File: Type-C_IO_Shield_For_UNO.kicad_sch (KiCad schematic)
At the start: 40 parts, among them J1 USB_C_Receptacle_USB2.0, J10 Conn_01x04, J11 Conn_01x04, J12 Conn_01x04, J13 Conn_01x04, J14 Conn_01x04, J15 Conn_01x04, J16 Conn_Alalog, J17 Conn_01x06, J18 Conn_01x06, J19 Conn_01x06, J2 Conn_01x04, J20 Conn_Digital, J21 Conn_01x04, J22 Conn_01x04, J23 Conn_IIC, J24 Conn_COM, J25 Conn_URF, J26 Conn_SD, J27 Conn_Bluetooth, J28 Screw_Terminal_01x02, J3 Conn_01x04, J4 Conn_01x04, J5 Conn_01x04, J6 Conn_01x04, J7 Conn_01x04, J8 Conn_Digital_2, J9 Conn_Power, U1 CH340C

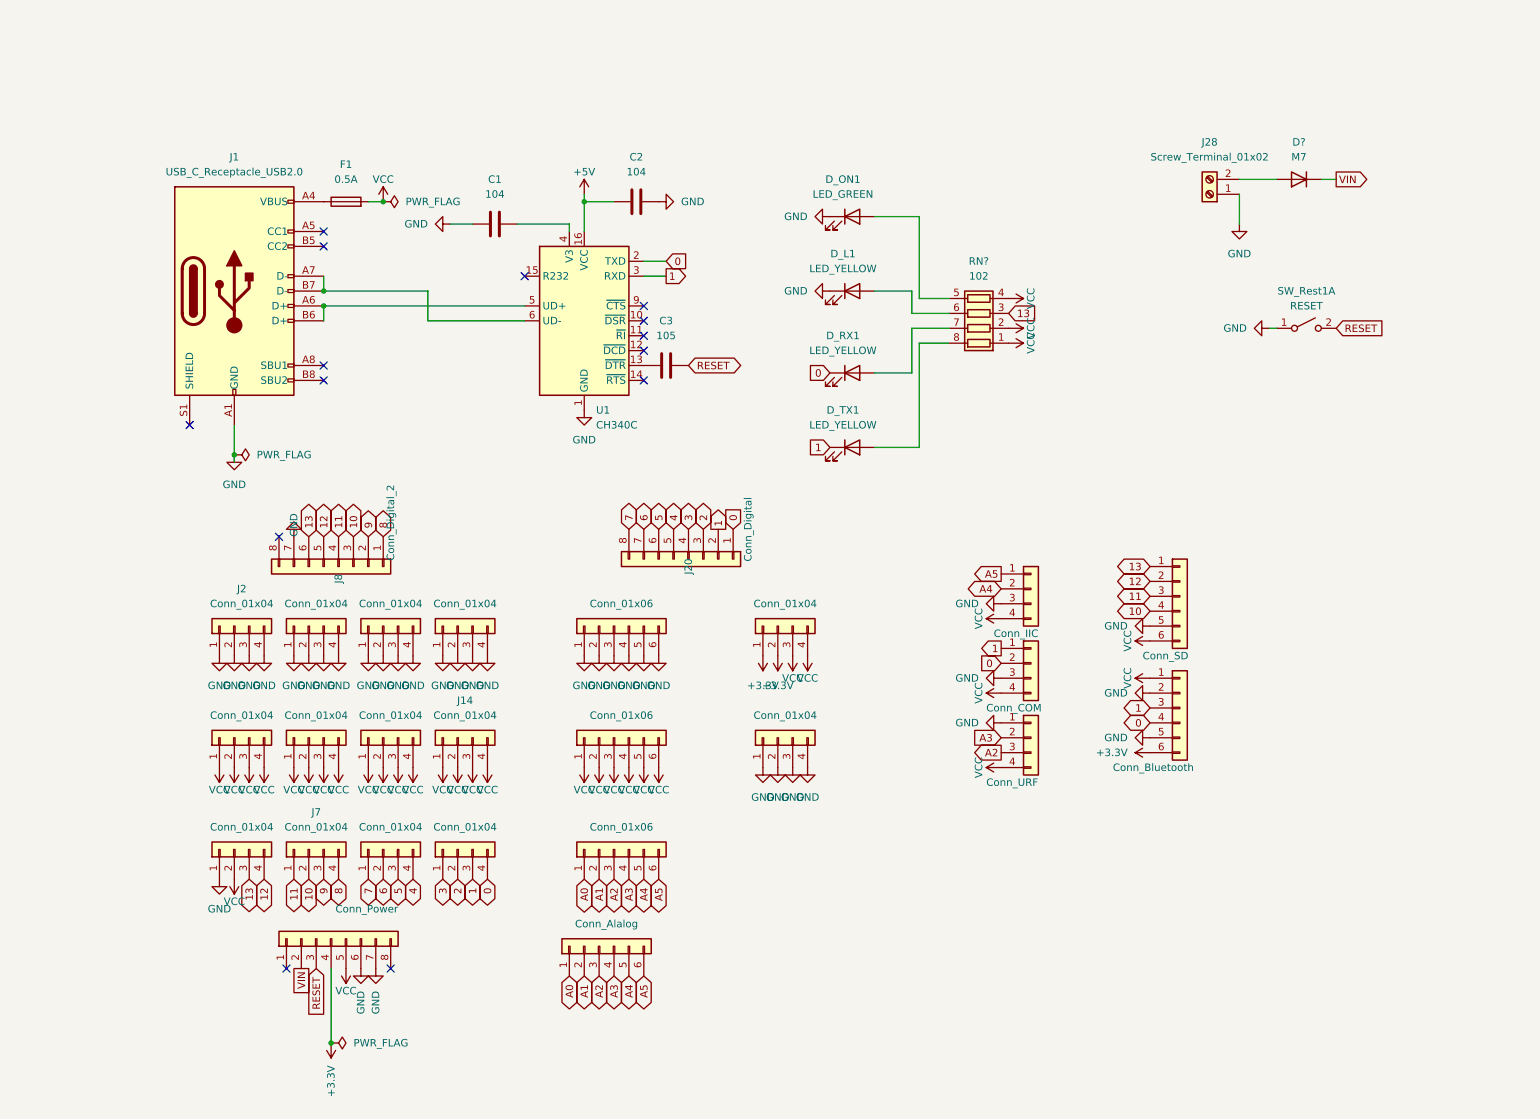
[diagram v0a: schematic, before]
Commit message: V1.1
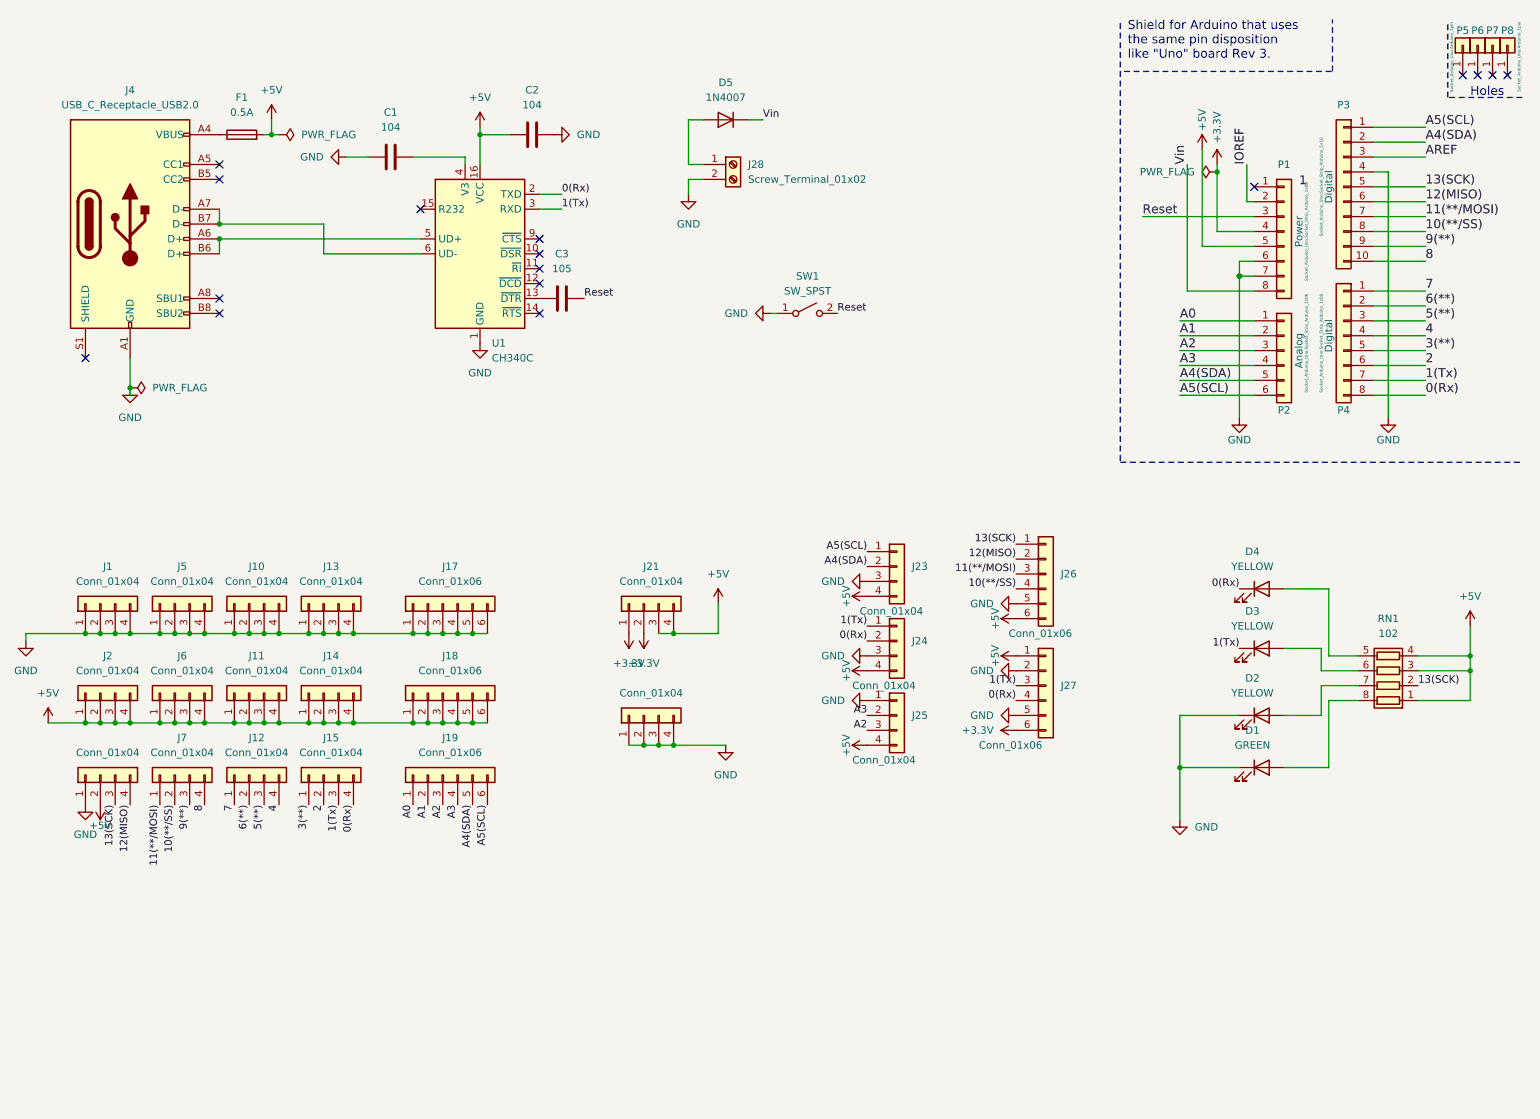
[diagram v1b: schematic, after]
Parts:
- removed D?: M7, Diode_SMD:D_SMA, symbol Diode:MRA4007T3G
- removed D_L1, D_RX1, D_TX1: LED_YELLOW, LED_SMD:LED_0805_2012Metric, symbol Device:LED
- removed D_ON1: LED_GREEN, LED_SMD:LED_0805_2012Metric, symbol Device:LED
- removed J1: USB_C_Receptacle_USB2.0, Connector_USB:USB_C_Receptacle_Palconn_UTC16-G, symbol Connector:USB_C_Receptacle_USB2.0
- removed J16: Conn_Alalog, Connector_PinSocket_2.54mm:PinSocket_1x06_P2.54mm_Vertical, symbol Connector_Generic:Conn_01x06
- removed J20: Conn_Digital, Connector_PinSocket_2.54mm:PinSocket_1x08_P2.54mm_Vertical, symbol Connector_Generic:Conn_01x08
- removed J4: Conn_01x04, Connector_PinHeader_2.54mm:PinHeader_1x04_P2.54mm_Vertical, symbol Connector_Generic:Conn_01x04
- removed J8: Conn_Digital_2, Connector_PinSocket_2.54mm:PinSocket_1x08_P2.54mm_Vertical, symbol Connector_Generic:Conn_01x08
- removed J9: Conn_Power, Connector_PinSocket_2.54mm:PinSocket_1x08_P2.54mm_Vertical, symbol Connector_Generic:Conn_01x08
- removed RN?: 102, Resistor_SMD:R_Array_Convex_4x1206, symbol Device:R_Pack04
- removed SW_Rest1: RESET, Button_Switch_SMD:SW_Push_1P1T_NO_CK_KSC6xxJ, symbol Switch:SW_DPST_x2
- added D1: GREEN, LED_SMD:LED_0805_2012Metric, symbol Device:LED
- added D2, D3, D4: YELLOW, LED_SMD:LED_0805_2012Metric, symbol Device:LED
- added D5: 1N4007, Diode_SMD:D_SMA, symbol Diode:1N4007
- added J1: Conn_01x04, Connector_PinHeader_2.54mm:PinHeader_1x04_P2.54mm_Vertical, symbol Connector_Generic:Conn_01x04
- added J4: USB_C_Receptacle_USB2.0, Connector_USB:USB_C_Receptacle_Palconn_UTC16-G, symbol Connector:USB_C_Receptacle_USB2.0
- added P1: Power, Socket_Arduino_Uno:Socket_Strip_Arduino_1x08, symbol Connector_Generic:Conn_01x08
- added P2: Analog, Socket_Arduino_Uno:Socket_Strip_Arduino_1x06, symbol Connector_Generic:Conn_01x06
- added P3: Digital, Socket_Arduino_Uno:Socket_Strip_Arduino_1x10, symbol Connector_Generic:Conn_01x10
- added P4: Digital, Socket_Arduino_Uno:Socket_Strip_Arduino_1x08, symbol Connector_Generic:Conn_01x08
- added P5, P6, P7, P8: CONN_01X01, Socket_Arduino_Uno:Arduino_1pin, symbol Connector_Generic:Conn_01x01
- added RN1: 102, Resistor_SMD:R_Array_Convex_4x1206, symbol Device:R_Pack04
- added SW1: SW_SPST, Button_Switch_SMD:SW_Push_1P1T_NO_6x6mm_H9.5mm, symbol Switch:SW_SPST
- J23: value Conn_IIC -> Conn_01x04
- J24: value Conn_COM -> Conn_01x04
- J25: value Conn_URF -> Conn_01x04
- J26: value Conn_SD -> Conn_01x06
- J27: value Conn_Bluetooth -> Conn_01x06
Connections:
- net +3V3: now also P1.4 (Pin_4)
- net 2: now also P4.6 (Pin_6)
- net 4: now also P4.4 (Pin_4)
- net 7: now also P4.1 (Pin_1)
- net 8: now also P3.10 (Pin_10)
- net A0: now also P2.1 (Pin_1)
- net A1: now also P2.2 (Pin_2)
- net A2: now also P2.3 (Pin_3)
- net A3: now also P2.4 (Pin_4)
- net GND: now also J28.2 (Pin_2), J3.1 (Pin_1), D1.1 (K), D2.1 (K), J1.1 (Pin_1), J1.2 (Pin_2), J1.3 (Pin_3), J1.4 (Pin_4), J4.A1 (GND), J4.A12 (GND), J4.B1 (GND), J4.B12 (GND), P1.6 (Pin_6), P1.7 (Pin_7), P3.4 (Pin_4), SW1.1 (A); no longer J2.1 (Pin_1), J2.2 (Pin_2), J2.3 (Pin_3), J2.4 (Pin_4), J28.1 (Pin_1)
- net at F1.1: now also J4.A4 (VBUS), J4.A9 (VBUS), J4.B4 (VBUS), J4.B9 (VBUS)
- net at U1.5 (UD+): now also J4.A6 (D+), J4.B6 (D+)
- net at U1.6 (UD-): now also J4.A7 (D-), J4.B7 (D-)
- net 0 renamed 0(Rx)
- net 0(Rx): now also D4.1 (K), P4.8 (Pin_8)
- net 1 renamed 1(Tx)
- net 1(Tx): now also D3.1 (K), P4.7 (Pin_7)
- net 10 renamed 10(**/SS)
- net 11 renamed 11(**/MOSI)
- net 12 renamed 12(MISO)
- net 12(MISO): now also J3.4 (Pin_4), P3.6 (Pin_6)
- net 13 renamed 13(SCK)
- net 13(SCK): now also J3.3 (Pin_3), P3.5 (Pin_5), RN1.2 (R2.1)
- net 3 renamed 3(**)
- net 3(**): now also P4.5 (Pin_5)
- net 5 renamed 5(**)
- net 5(**): now also P4.3 (Pin_3)
- net 6 renamed 6(**)
- net 6(**): now also P4.2 (Pin_2)
- net 9 renamed 9(**)
- net 9(**): now also P3.9 (Pin_9)
- net A4 renamed A4(SDA)
- net A4(SDA): now also P2.5 (Pin_5), P3.2 (Pin_2)
- net A5 renamed A5(SCL)
- net A5(SCL): now also P2.6 (Pin_6), P3.1 (Pin_1)
- net RESET renamed Reset
- net Reset: now also P1.3 (Pin_3), SW1.2 (B)
- net VCC renamed +5V
- net +5V: now also J2.1 (Pin_1), J2.2 (Pin_2), J2.3 (Pin_3), J2.4 (Pin_4), P1.5 (Pin_5), RN1.1 (R1.1), RN1.3 (R3.1), RN1.4 (R4.1); no longer J3.1 (Pin_1), J3.3 (Pin_3), J3.4 (Pin_4)
- new net: D2.2 (A), RN1.7 (R2.2)
- new net: D4.2 (A), RN1.5 (R4.2)
- new net: D3.2 (A), RN1.6 (R3.2)
- new net: D1.2 (A), RN1.8 (R1.2)
- new net: D5.2 (A), J28.1 (Pin_1)
- new net 10(**/SS): P3.8 (Pin_8)
- new net 11(**/MOSI): P3.7 (Pin_7)
- new net AREF: P3.3 (Pin_3)
- new net IOREF: P1.2 (Pin_2)
- new net Vin: D5.1 (K), P1.8 (Pin_8)
- no-connect marks 14 -> 16
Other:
- note added: "1"
- note added: "Holes"
- note added: "Shield for Arduino that uses the same pin disposition like "Uno" board Rev 3."
